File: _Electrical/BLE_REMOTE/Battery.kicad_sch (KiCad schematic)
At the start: 29 parts, among them J4 Battery, Q1 IRLML6244, Q1 RE1C002UNTCL, Q2 IRLML6244, SW1 SW_Push, U3 IRF7319TRPBF, U3 MCP65R41

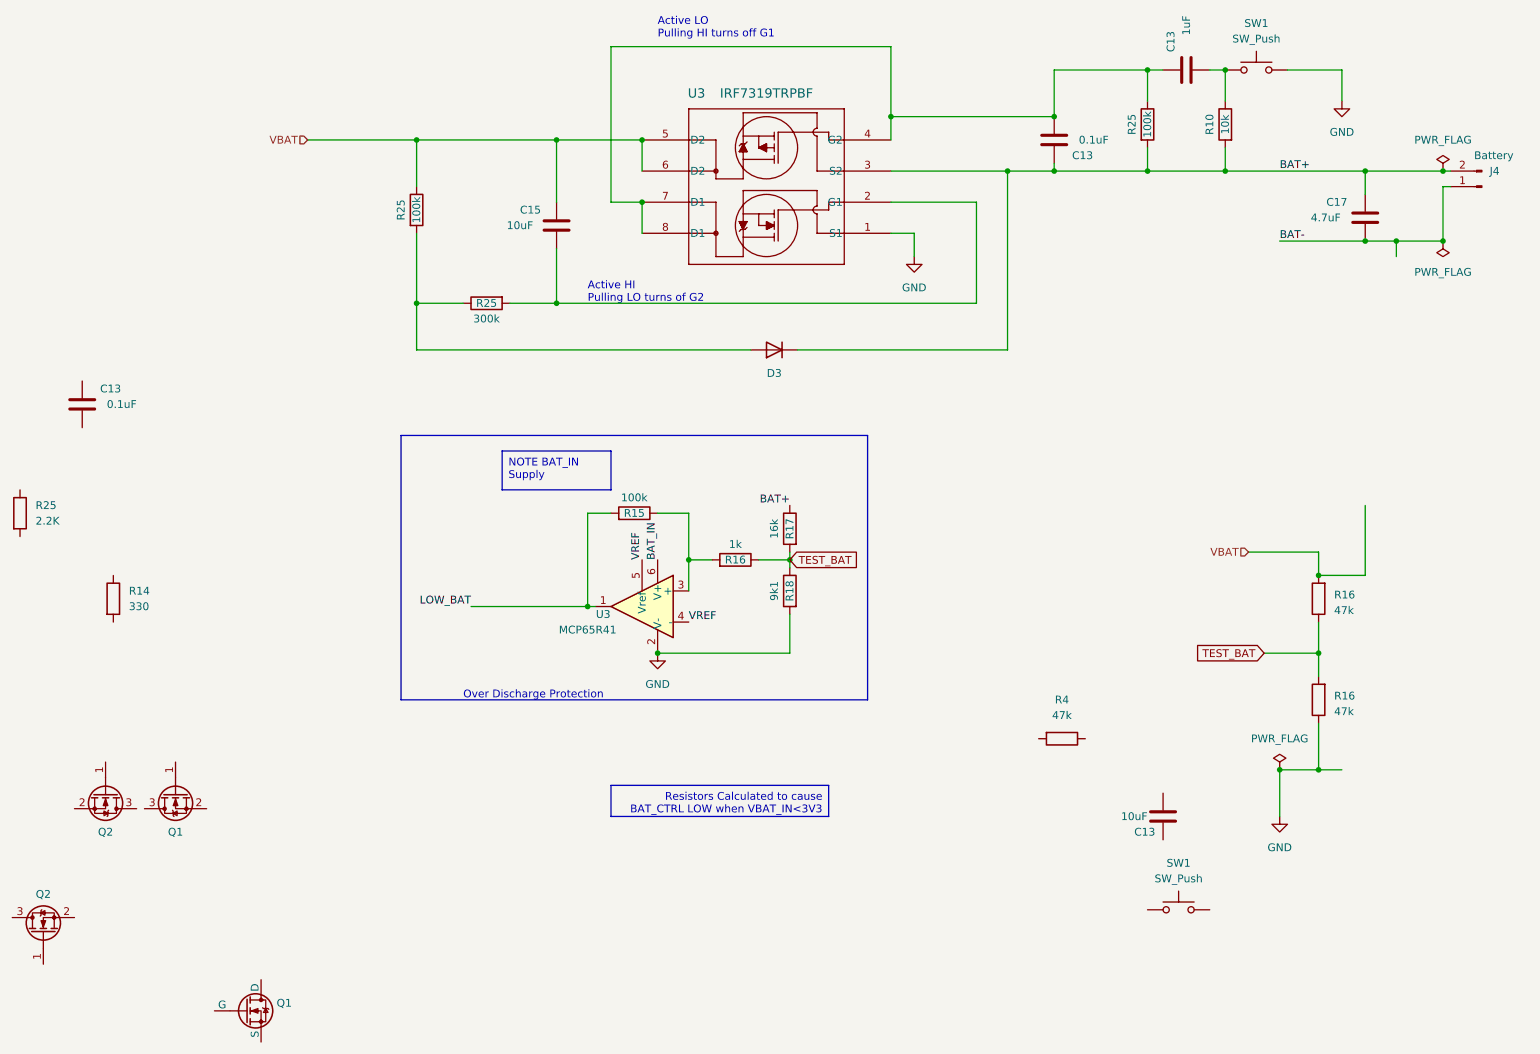
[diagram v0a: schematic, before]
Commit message: started PCB design
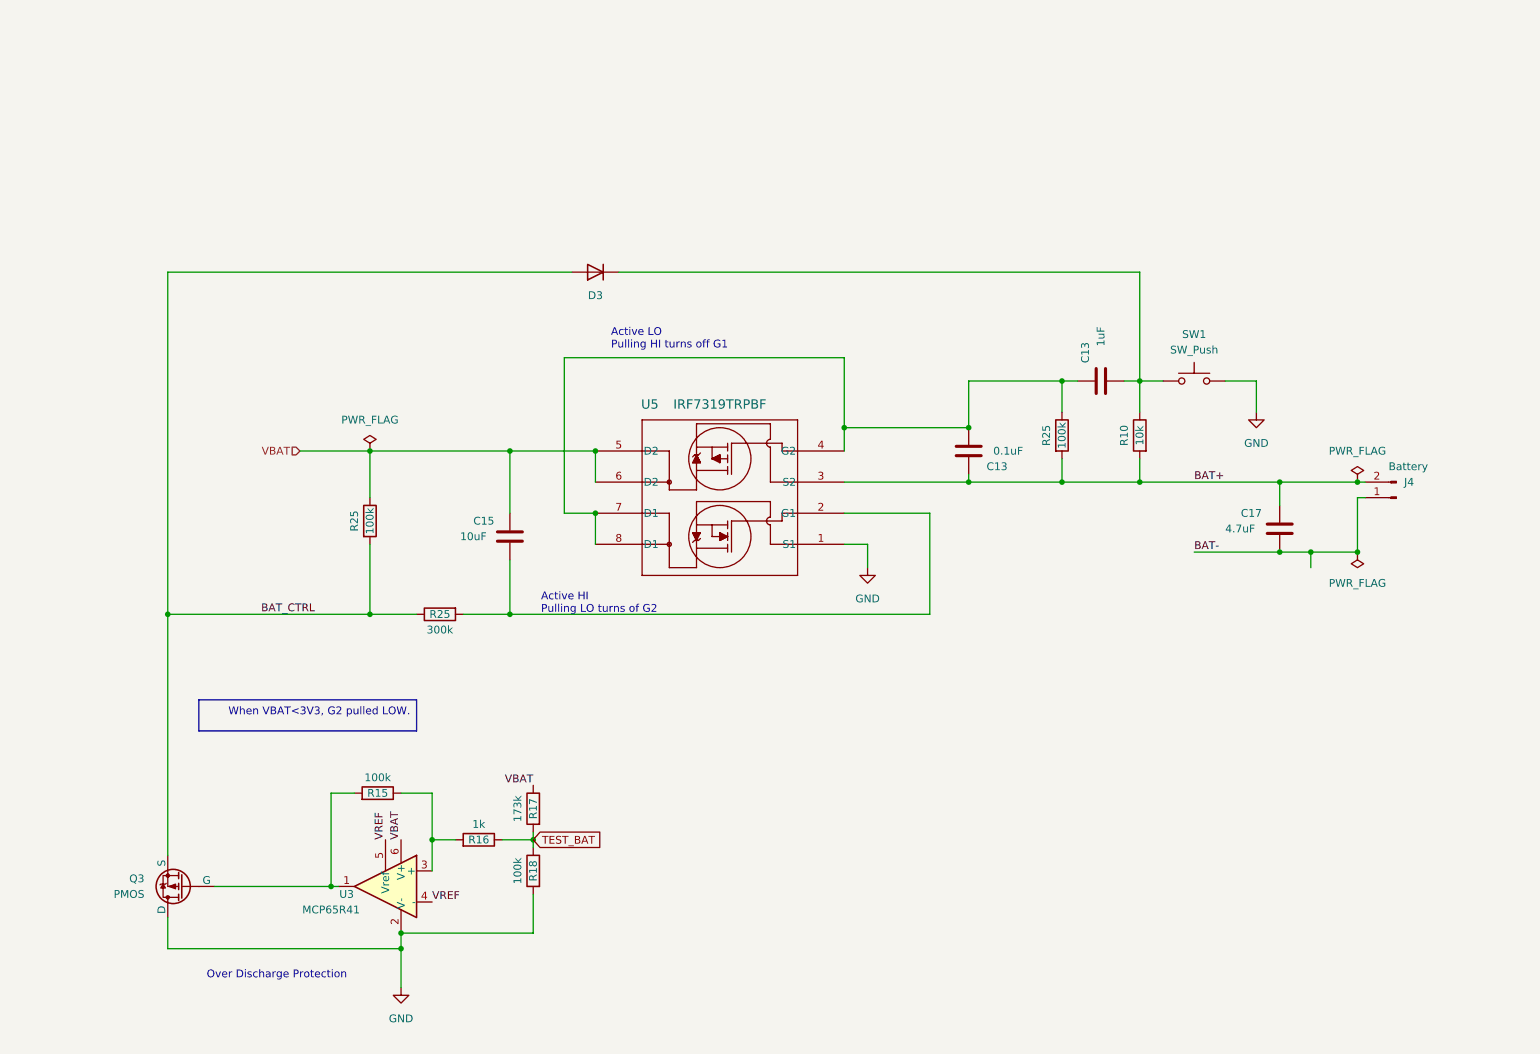
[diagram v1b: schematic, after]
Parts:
- removed C13: 0.1uF, Capacitor_SMD:C_0402_1005Metric_Pad0.74x0.62mm_HandSolder, symbol Device:C
- removed C13: 10uF, Capacitor_SMD:C_0402_1005Metric_Pad0.74x0.62mm_HandSolder, symbol Device:C
- removed Q1, Q2 (x2): IRLML6244, Package_TO_SOT_SMD:SOT-23, symbol Transistor_FET:IRLML6244
- removed Q1: RE1C002UNTCL, _Parts:DIO_RB558WMF_ROM, symbol Simulation_SPICE:NMOS
- removed R14: 330, Resistor_SMD:R_0402_1005Metric_Pad0.72x0.64mm_HandSolder, symbol Device:R
- removed R16 (x2), R4: 47k, Resistor_SMD:R_0402_1005Metric_Pad0.72x0.64mm_HandSolder, symbol Device:R
- removed R25: 2.2K, Resistor_SMD:R_0402_1005Metric_Pad0.72x0.64mm_HandSolder, symbol Device:R
- removed SW1: SW_Push, symbol Switch:SW_Push
- added Q3: PMOS, Package_TO_SOT_SMD:SOT-323_SC-70_Handsoldering, symbol Simulation_SPICE:PMOS
- R17: value 16k -> 173k
- R18: value 9k1 -> 100k
- SW1: footprint (none) -> Button_Switch_SMD:SW_Push_1P1T_NO_6x6mm_H9.5mm
- renumbered U3 to U5
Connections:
- net BAT_IN is gone; now on net VBAT: U3.6 (V+)
- net BAT+: no longer D3.1 (K), R17.1
- net GND: now also Q3.1 (D)
- net VBAT: now also R17.1
- net at C13.2, R10.1, SW1.1: now also D3.1 (K)
- net BAT_CTRL: now reaches D3.2 (A), R25.1, R25.2
- net BAT_CTRL: now also Q3.3 (S)
- net LOW_BAT: no longer names the net of R15.2, U3.1
- net LOW_BAT: now also Q3.2 (G)
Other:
- moved on the sheet: C13, C15, C17, D3, J4, R10, R15, R16, R17, R18, R25, SW1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
